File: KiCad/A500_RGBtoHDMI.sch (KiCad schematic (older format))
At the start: 3 parts, among them J1 Conn_02x20_Odd_Even, U1 Denise_MB_pins, U2 Denise_SocketOnAdapter

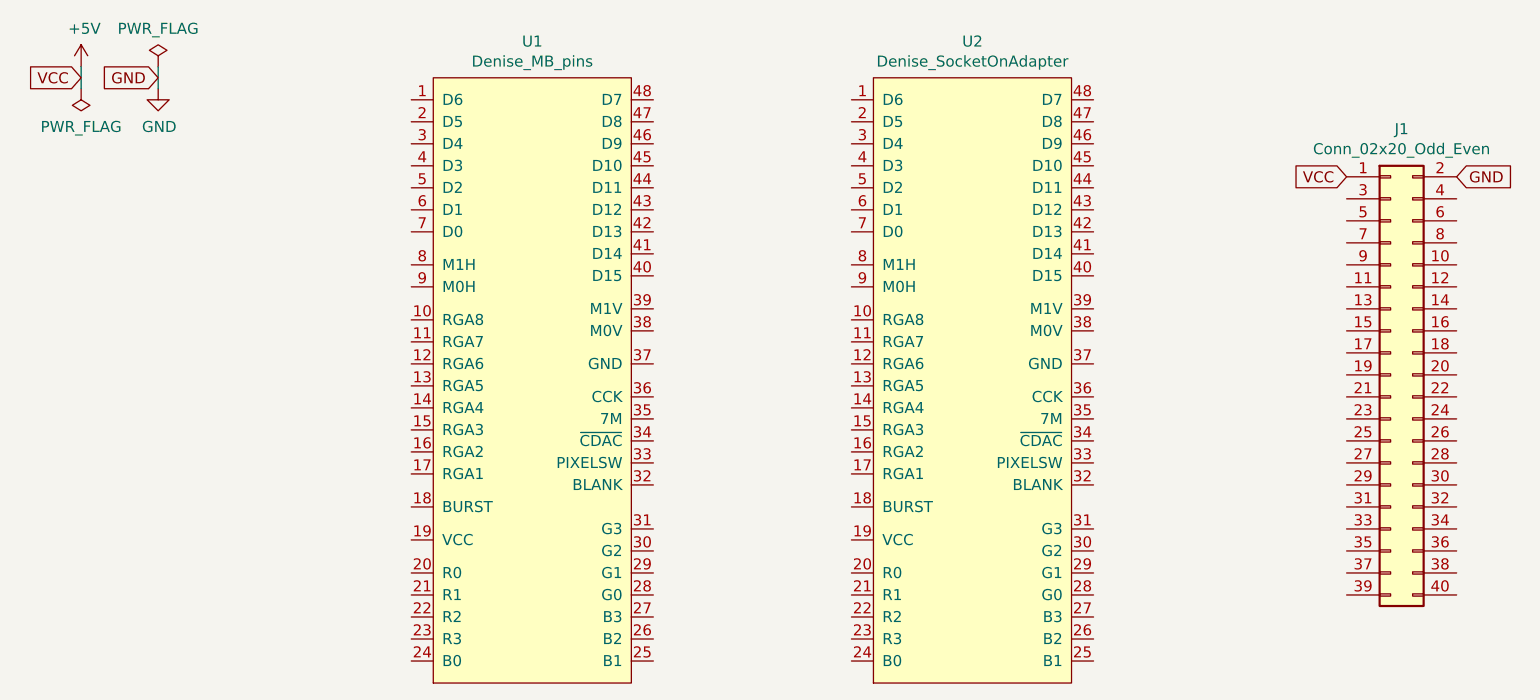
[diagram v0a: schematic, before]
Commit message: improved design
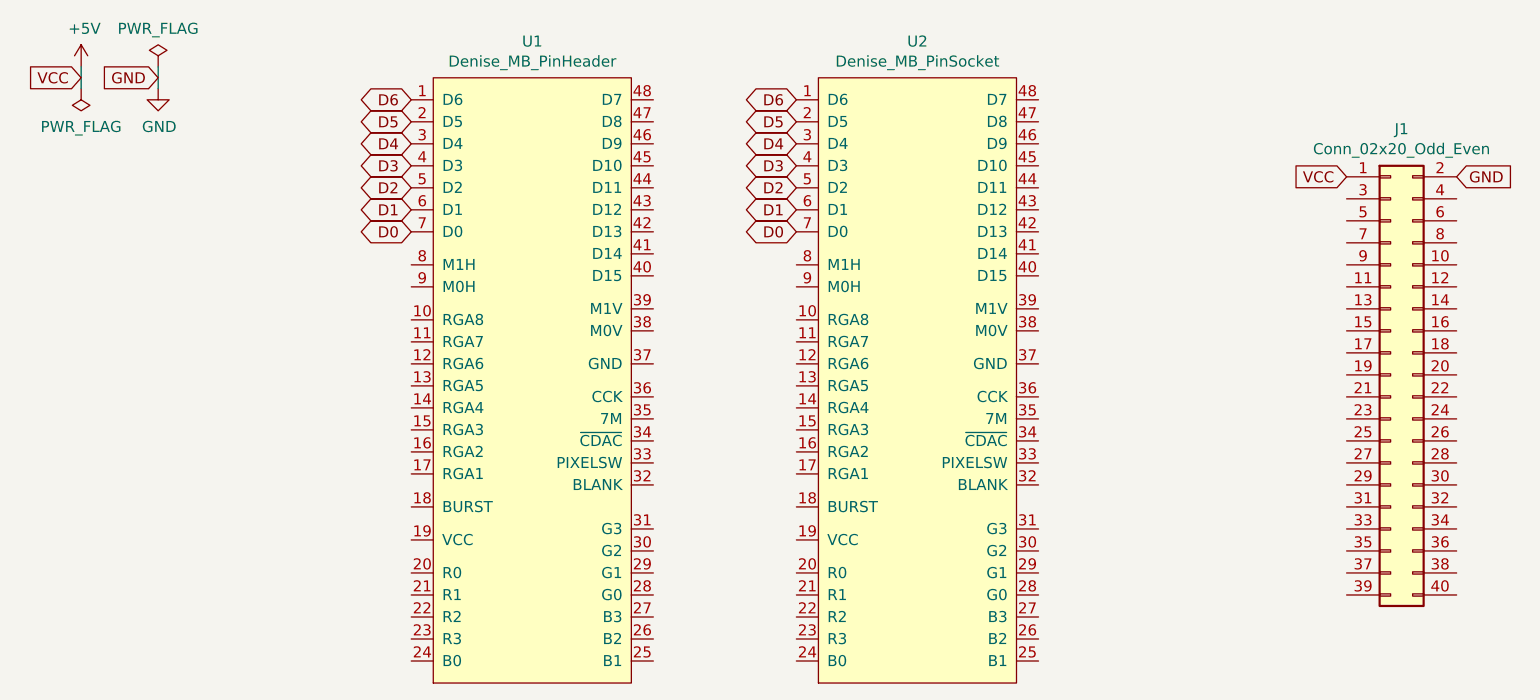
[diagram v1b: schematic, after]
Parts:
- U1: value Denise_MB_pins -> Denise_MB_PinHeader
- U2: value Denise_SocketOnAdapter -> Denise_MB_PinSocket
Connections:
- net D6: now reaches U1.1 (D6)
- net D6: now also U2.1 (D6)
- net D5: now reaches U1.2 (D5)
- net D5: now also U2.2 (D5)
- net D4: now reaches U1.3 (D4)
- net D4: now also U2.3 (D4)
- net D3: now reaches U1.4 (D3)
- net D3: now also U2.4 (D3)
- net D2: now reaches U1.5 (D2)
- net D2: now also U2.5 (D2)
- net D1: now reaches U1.6 (D1)
- net D1: now also U2.6 (D1)
- net D0: now reaches U1.7 (D0)
- net D0: now also U2.7 (D0)
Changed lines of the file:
@@
 P 2950 3100
 F 0 "U1" H 2950 4665 50  0000 C CNN
-F 1 "Denise_MB_pins" H 2950 4574 50  0000 C CNN
+F 1 "Denise_MB_PinHeader" H 2950 4574 50  0000 C CNN
 F 2 "Package_DIP:DIP-48_W15.24mm_LongPads" H 2900 1600 50  0001 C CNN
 F 3 "" H 2900 1600 50  0001 C CNN
@@
 $Comp
 L A500_RGBtoHDMI:Denise U2
-U 1 1 623C9B51
-P 4950 3100
-F 0 "U2" H 4950 4665 50  0000 C CNN
-F 1 "Denise_SocketOnAdapter" H 4950 4574 50  0000 C CNN
-F 2 "Package_DIP:DIP-48_W15.24mm_Socket_LongPads" H 4900 1600 50  0001 C CNN
-F 3 "" H 4900 1600 50  0001 C CNN
-	1    4950 3100
+U 1 1 623E379A
+P 4700 3100
+F 0 "U2" H 4700 4665 50  0000 C CNN
+F 1 "Denise_MB_PinSocket" H 4700 4574 50  0000 C CNN
+F 2 "Package_DIP:DIP-48_W15.24mm_Socket_LongPads" H 4650 1600 50  0001 C CNN
+F 3 "" H 4650 1600 50  0001 C CNN
+	1    4700 3100
 	1    0    0    -1
 $EndComp
+Text GLabel 2400 1800 0    50   BiDi ~ 0
+D6
+Text GLabel 4150 1800 0    50   BiDi ~ 0
+D6
+Text GLabel 2400 1900 0    50   BiDi ~ 0
+D5
+Text GLabel 4150 1900 0    50   BiDi ~ 0
+D5
+Text GLabel 2400 2000 0    50   BiDi ~ 0
+D4
+Text GLabel 2400 2100 0    50   BiDi ~ 0
+D3
+Text GLabel 2400 2200 0    50   BiDi ~ 0
+D2
+Text GLabel 2400 2300 0    50   BiDi ~ 0
+D1
+Text GLabel 2400 2400 0    50   BiDi ~ 0
+D0
+Text GLabel 4150 2000 0    50   BiDi ~ 0
+D4
+Text GLabel 4150 2100 0    50   BiDi ~ 0
+D3
+Text GLabel 4150 2200 0    50   BiDi ~ 0
+D2
+Text GLabel 4150 2300 0    50   BiDi ~ 0
+D1
+Text GLabel 4150 2400 0    50   BiDi ~ 0
+D0
 $EndSCHEMATC

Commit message: more routing
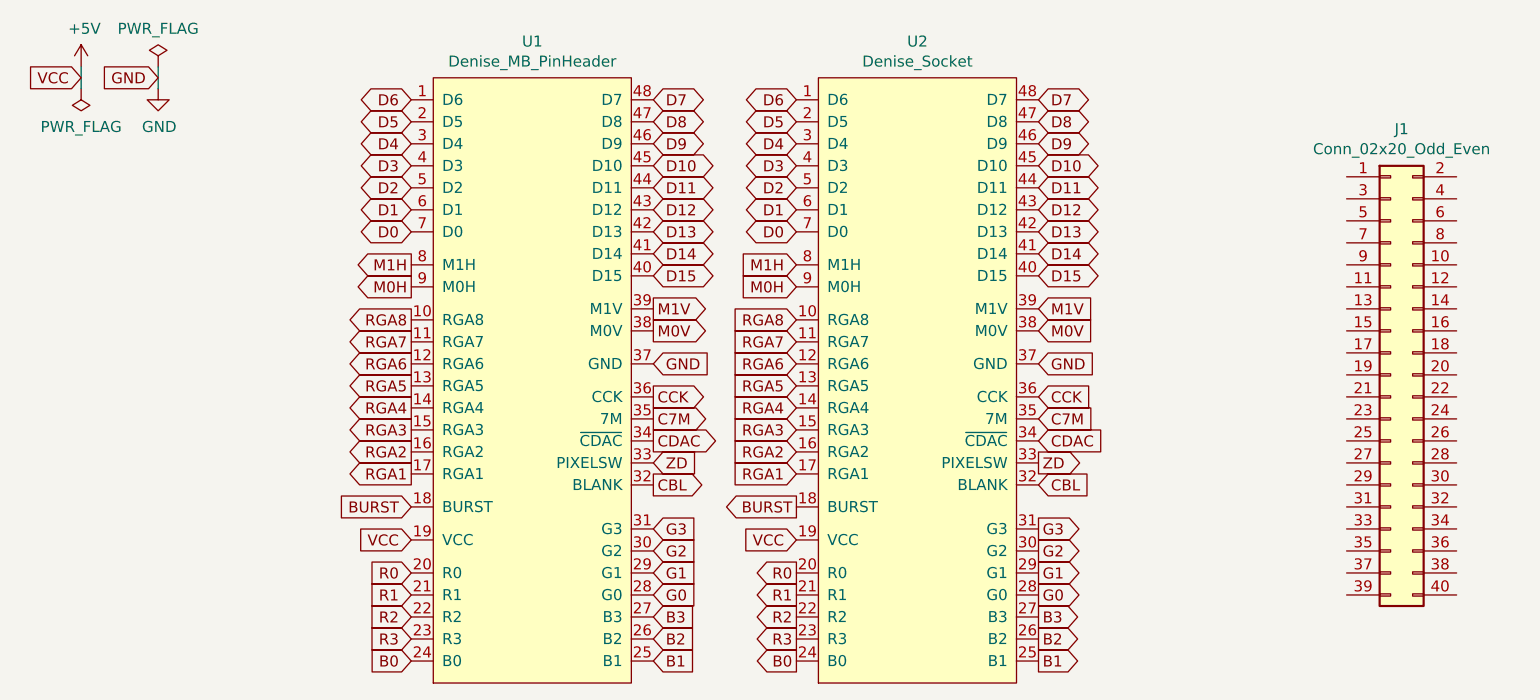
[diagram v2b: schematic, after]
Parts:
- U2: value Denise_MB_PinSocket -> Denise_Socket
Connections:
- net +5V: now also U1.19 (VCC), U2.19 (VCC); no longer J1.1 (Pin_1)
- net GND: now also U1.37 (GND), U2.37 (GND); no longer J1.2 (Pin_2)
- net RGA8: now reaches U1.10 (RGA8)
- net RGA8: now also U2.10 (RGA8)
- net RGA7: now reaches U1.11 (RGA7)
- net RGA7: now also U2.11 (RGA7)
- net RGA6: now reaches U1.12 (RGA6)
- net RGA6: now also U2.12 (RGA6)
- net RGA5: now reaches U1.13 (RGA5)
- net RGA5: now also U2.13 (RGA5)
- net RGA4: now reaches U1.14 (RGA4)
- net RGA4: now also U2.14 (RGA4)
- net RGA3: now reaches U1.15 (RGA3)
- net RGA3: now also U2.15 (RGA3)
- net RGA2: now reaches U1.16 (RGA2)
- net RGA2: now also U2.16 (RGA2)
- net RGA1: now reaches U1.17 (RGA1)
- net RGA1: now also U2.17 (RGA1)
- net BURST: now reaches U1.18 (BURST)
- net BURST: now also U2.18 (BURST)
- net R0: now reaches U1.20 (R0)
- net R0: now also U2.20 (R0)
- net R1: now reaches U1.21 (R1)
- net R1: now also U2.21 (R1)
- net R2: now reaches U1.22 (R2)
- net R2: now also U2.22 (R2)
- net R3: now reaches U1.23 (R3)
- net R3: now also U2.23 (R3)
- net B0: now reaches U1.24 (B0)
- net B0: now also U2.24 (B0)
- net B1: now reaches U1.25 (B1)
- net B1: now also U2.25 (B1)
- net B2: now reaches U1.26 (B2)
- net B2: now also U2.26 (B2)
- net B3: now reaches U1.27 (B3)
- net B3: now also U2.27 (B3)
- net G0: now reaches U1.28 (G0)
- net G0: now also U2.28 (G0)
- net G1: now reaches U1.29 (G1)
- net G1: now also U2.29 (G1)
- net G2: now reaches U1.30 (G2)
- net G2: now also U2.30 (G2)
- net G3: now reaches U1.31 (G3)
- net G3: now also U2.31 (G3)
- net CBL: now reaches U1.32 (BLANK)
- net CBL: now also U2.32 (BLANK)
- net ZD: now reaches U1.33 (PIXELSW)
- net ZD: now also U2.33 (PIXELSW)
- net CDAC: now reaches U1.34 (~CDAC)
- net CDAC: now also U2.34 (~CDAC)
- net C7M: now reaches U1.35 (7M)
- net C7M: now also U2.35 (7M)
- net CCK: now reaches U1.36 (CCK)
- net CCK: now also U2.36 (CCK)
- net M0V: now reaches U1.38 (M0V)
- net M0V: now also U2.38 (M0V)
- net M1V: now reaches U1.39 (M1V)
- net M1V: now also U2.39 (M1V)
- net D15: now reaches U1.40 (D15)
- net D15: now also U2.40 (D15)
- net D14: now reaches U1.41 (D14)
- net D14: now also U2.41 (D14)
- net D13: now reaches U1.42 (D13)
- net D13: now also U2.42 (D13)
- net D12: now reaches U1.43 (D12)
- net D12: now also U2.43 (D12)
- net D11: now reaches U1.44 (D11)
- net D11: now also U2.44 (D11)
- net D10: now reaches U1.45 (D10)
- net D10: now also U2.45 (D10)
- net D9: now reaches U1.46 (D9)
- net D9: now also U2.46 (D9)
- net D8: now reaches U1.47 (D8)
- net D8: now also U2.47 (D8)
- net D7: now reaches U1.48 (D7)
- net D7: now also U2.48 (D7)
- net M1H: now reaches U1.8 (M1H)
- net M1H: now also U2.8 (M1H)
- net M0H: now reaches U1.9 (M0H)
- net M0H: now also U2.9 (M0H)
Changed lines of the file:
@@
 	1    0    0    -1
 $EndComp
-Text GLabel 6650 2150 0    50   Input ~ 0
-VCC
-Text GLabel 7150 2150 2    50   Input ~ 0
-GND
 $Comp
 L A500_RGBtoHDMI:Denise U1
@@
 P 4700 3100
 F 0 "U2" H 4700 4665 50  0000 C CNN
-F 1 "Denise_MB_PinSocket" H 4700 4574 50  0000 C CNN
+F 1 "Denise_Socket" H 4700 4574 50  0000 C CNN
 F 2 "Package_DIP:DIP-48_W15.24mm_Socket_LongPads" H 4650 1600 50  0001 C CNN
 F 3 "" H 4650 1600 50  0001 C CNN
@@
 Text GLabel 4150 2400 0    50   BiDi ~ 0
 D0
+Text GLabel 2400 2550 0    50   Output ~ 0
+M1H
+Text GLabel 2400 2650 0    50   Output ~ 0
+M0H
+Text GLabel 4150 2550 0    50   Input ~ 0
+M1H
+Text GLabel 4150 2650 0    50   Input ~ 0
+M0H
+Text GLabel 2400 3000 0    50   Output ~ 0
+RGA6
+Text GLabel 2400 3100 0    50   Output ~ 0
+RGA5
+Text GLabel 2400 3200 0    50   Output ~ 0
+RGA4
+Text GLabel 2400 3300 0    50   Output ~ 0
+RGA3
+Text GLabel 2400 3400 0    50   Output ~ 0
+RGA2
+Text GLabel 2400 3500 0    50   Output ~ 0
+RGA1
+Text GLabel 2400 2900 0    50   Output ~ 0
+RGA7
+Text GLabel 2400 2800 0    50   Output ~ 0
+RGA8
+Text GLabel 4150 3000 0    50   Input ~ 0
+RGA6
+Text GLabel 4150 3100 0    50   Input ~ 0
+RGA5
+Text GLabel 4150 3200 0    50   Input ~ 0
+RGA4
+Text GLabel 4150 3300 0    50   Input ~ 0
+RGA3
+Text GLabel 4150 3400 0    50   Input ~ 0
+RGA2
+Text GLabel 4150 3500 0    50   Input ~ 0
+RGA1
+Text GLabel 4150 2900 0    50   Input ~ 0
+RGA7
+Text GLabel 4150 2800 0    50   Input ~ 0
+RGA8
+Text GLabel 4150 3650 0    50   Output ~ 0
+BURST
+Text GLabel 2400 3650 0    50   Input ~ 0
+BURST
+Text GLabel 2400 3800 0    50   Input ~ 0
+VCC
+Text GLabel 4150 3800 0    50   Input ~ 0
+VCC
+Text GLabel 2400 4050 0    50   Input ~ 0
+R1
+Text GLabel 2400 3950 0    50   Input ~ 0
+R0
+Text GLabel 2400 4250 0    50   Input ~ 0
+R3
+Text GLabel 2400 4150 0    50   Input ~ 0
+R2
+Text GLabel 2400 4350 0    50   Input ~ 0
+B0
+Text GLabel 4150 4050 0    50   Output ~ 0
+R1
+Text GLabel 4150 3950 0    50   Output ~ 0
+R0
+Text GLabel 4150 4250 0    50   Output ~ 0
+R3
+Text GLabel 4150 4150 0    50   Output ~ 0
+R2
+Text GLabel 4150 4350 0    50   Output ~ 0
+B0
+Text GLabel 3500 3950 2    50   Input ~ 0
+G1
+Text GLabel 3500 4050 2    50   Input ~ 0
+G0
+Text GLabel 3500 4250 2    50   Input ~ 0
+B2
+Text GLabel 3500 4150 2    50   Input ~ 0
+B3
+Text GLabel 3500 4350 2    50   Input ~ 0
+B1
+Text GLabel 3500 3750 2    50   Input ~ 0
+G3
+Text GLabel 3500 3850 2    50   Input ~ 0
+G2
+Text GLabel 5250 3950 2    50   Output ~ 0
+G1
+Text GLabel 5250 4050 2    50   Output ~ 0
+G0
+Text GLabel 5250 4250 2    50   Output ~ 0
+B2
+Text GLabel 5250 4150 2    50   Output ~ 0
+B3
+Text GLabel 5250 4350 2    50   Output ~ 0
+B1
+Text GLabel 5250 3750 2    50   Output ~ 0
+G3
+Text GLabel 5250 3850 2    50   Output ~ 0
+G2
+Text GLabel 5250 3550 2    50   Input ~ 0
+CBL
+Text GLabel 3500 3550 2    50   Output ~ 0
+CBL
+Text GLabel 5250 3450 2    50   Output ~ 0
+ZD
+Text GLabel 3500 3450 2    50   Input ~ 0
+ZD
+Text GLabel 5250 3350 2    50   Input ~ 0
+CDAC
+Text GLabel 3500 3350 2    50   Output ~ 0
+CDAC
+Text GLabel 3500 3250 2    50   Output ~ 0
+C7M
+Text GLabel 5250 3250 2    50   Input ~ 0
+C7M
+Text GLabel 3500 3150 2    50   Output ~ 0
+CCK
+Text GLabel 5250 3150 2    50   Input ~ 0
+CCK
+Text GLabel 3500 3000 2    50   Input ~ 0
+GND
+Text GLabel 5250 3000 2    50   Input ~ 0
+GND
+Text GLabel 3500 2750 2    50   Output ~ 0
+M1V
+Text GLabel 3500 2850 2    50   Output ~ 0
+M0V
+Text GLabel 5250 2750 2    50   Input ~ 0
+M1V
+Text GLabel 5250 2850 2    50   Input ~ 0
+M0V
+Text GLabel 3500 1800 2    50   BiDi ~ 0
+D7
+Text GLabel 3500 1900 2    50   BiDi ~ 0
+D8
+Text GLabel 3500 2000 2    50   BiDi ~ 0
+D9
+Text GLabel 3500 2100 2    50   BiDi ~ 0
+D10
+Text GLabel 3500 2200 2    50   BiDi ~ 0
+D11
+Text GLabel 3500 2300 2    50   BiDi ~ 0
+D12
+Text GLabel 3500 2400 2    50   BiDi ~ 0
+D13
+Text GLabel 3500 2500 2    50   BiDi ~ 0
+D14
+Text GLabel 3500 2600 2    50   BiDi ~ 0
+D15
+Text GLabel 5250 1800 2    50   BiDi ~ 0
+D7
+Text GLabel 5250 1900 2    50   BiDi ~ 0
+D8
+Text GLabel 5250 2000 2    50   BiDi ~ 0
+D9
+Text GLabel 5250 2100 2    50   BiDi ~ 0
+D10
+Text GLabel 5250 2200 2    50   BiDi ~ 0
+D11
+Text GLabel 5250 2300 2    50   BiDi ~ 0
+D12
+Text GLabel 5250 2400 2    50   BiDi ~ 0
+D13
+Text GLabel 5250 2500 2    50   BiDi ~ 0
+D14
+Text GLabel 5250 2600 2    50   BiDi ~ 0
+D15
 $EndSCHEMATC
